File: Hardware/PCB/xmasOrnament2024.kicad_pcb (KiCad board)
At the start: 2 copper layers, 60 x 66.9 mm, 55 parts, among them IC1 TP4056-42, Q1 AO3401A, Q2 CJ3400, SW1 BZCN_TSA007A1518B03, SW2 BZCN_TSA007A1518B03, U1 STM32C011F6

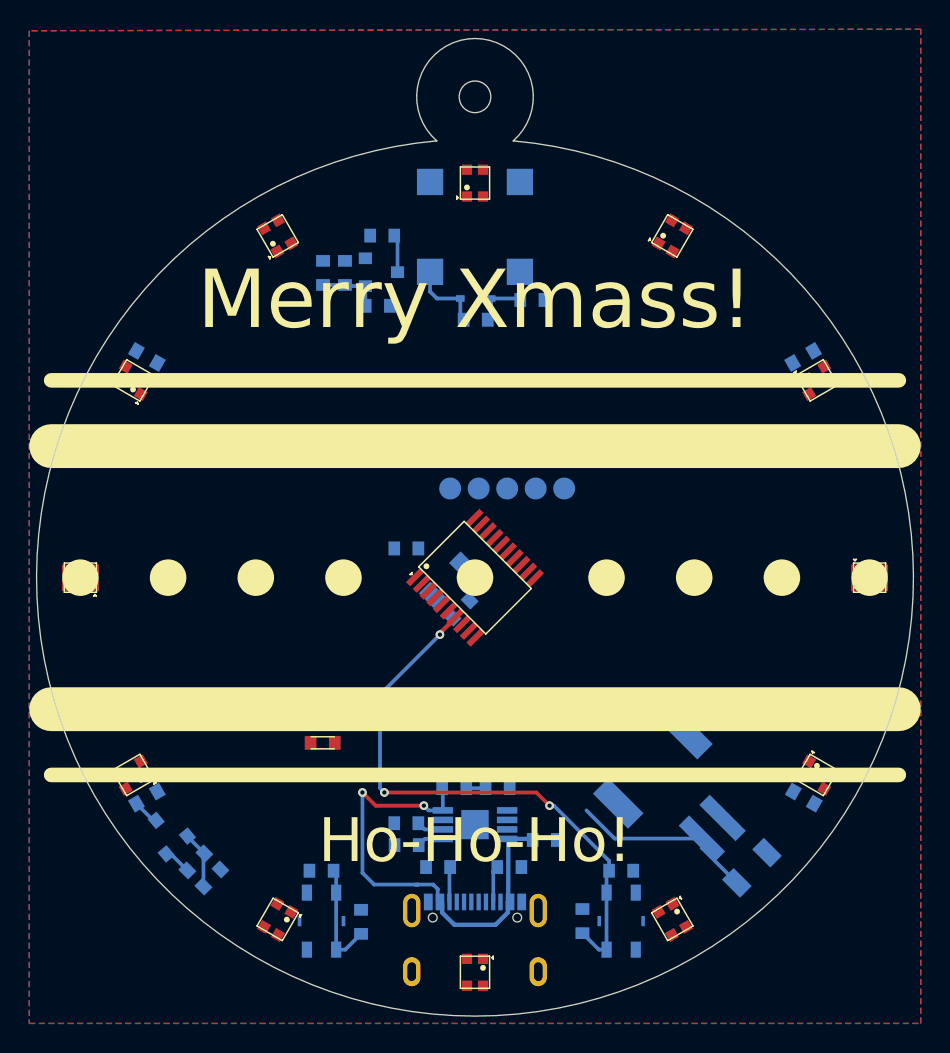
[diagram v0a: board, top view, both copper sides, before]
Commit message: Board finished.
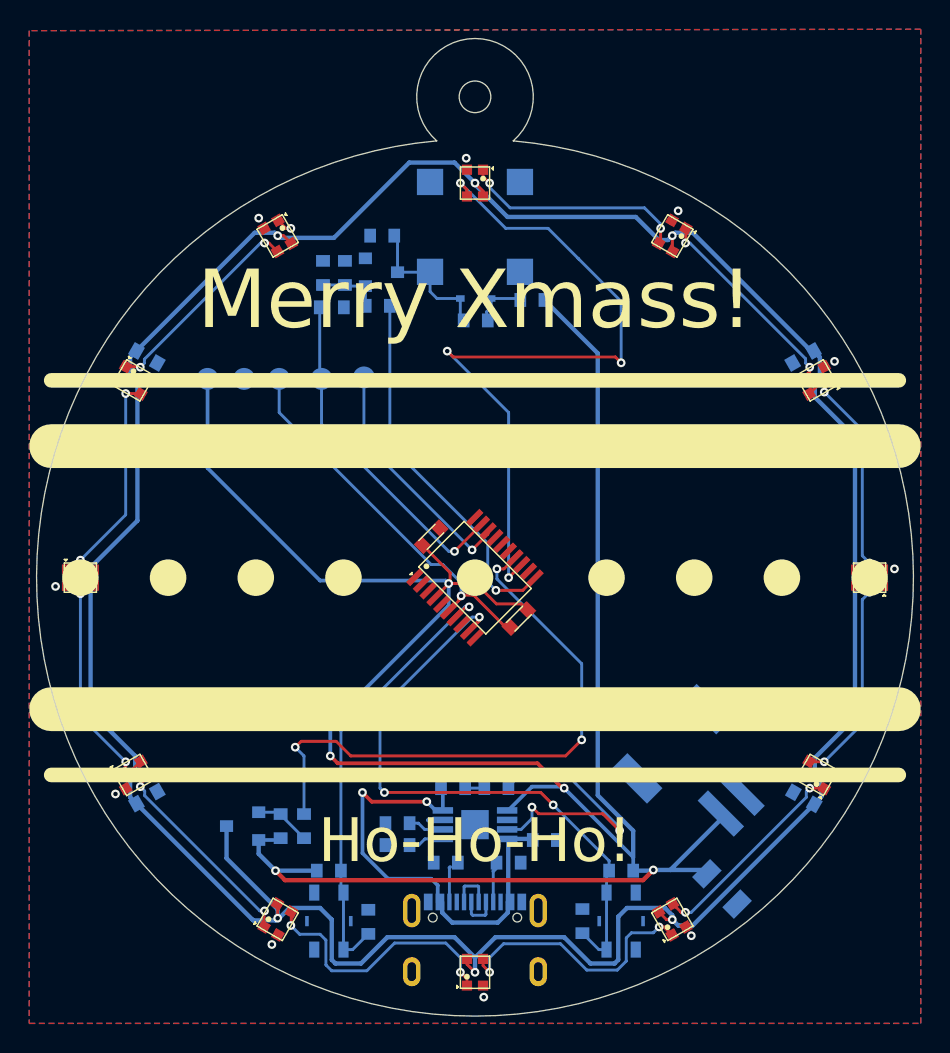
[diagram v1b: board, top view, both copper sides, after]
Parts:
- C4, R13: moved to F.Cu
- R14: moved to B.Cu
- moved R14 29.8 mm to (134.1, 77.2)
- moved TP5 20.9 mm to (130.4, 82.1)
- moved TP2 18.2 mm to (125.5, 82.1)
- moved TP1 17.7 mm to (128.1, 82.1)
- moved TP3 14.7 mm to (133.3, 82.1)
- moved TP4 14.0 mm to (136.2, 82.0)
- moved C3 13.3 mm to (132.3, 105.1), turned to 0 degrees
- moved R7 7.23 mm to (132.2, 112.7), turned to 90 degrees
- moved R6 6.30 mm to (130.6, 112.7), turned to 90 degrees
- moved Q1 5.23 mm to (128.0, 112.7), turned to -90 degrees
- moved R13 4.00 mm to (146.8, 98.5)
- moved C1 2.51 mm to (160.8, 117.0), turned to 135 degrees
- moved CONN1 2.15 mm to (161.4, 111.1)
- moved C4 1.88 mm to (140.8, 92.9), turned to -135 degrees
- moved R2 0.62 mm to (138.6, 114.0)
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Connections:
- C1 pad 2: Net-(IC1-BAT) -> VDD
- CONN1 pad +: Net-(IC1-BAT) -> VDD
- IC1 pad 5: Net-(IC1-BAT) -> VDD
- U1 pad 7: /BTN1 -> /BTN2
- U1 pad 9: /BTN2 -> /BTN1
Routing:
- net WS_SUPPLY: track 1.80 -> 215.0 mm, vias 0 -> 12
- net VDD: track 1.77 -> 165.6 mm, vias 0 -> 5
- net /WS_DIN: track 0.00 -> 50.4 mm, vias 0 -> 4
- net /PERIPH_SUPPLY: track 0.00 -> 41.1 mm, vias 0 -> 3
- net /RST: track 0.00 -> 26.3 mm, vias 0 -> 1
- net /BUZZER: track 0.00 -> 25.5 mm, vias 0 -> 1
- net /SW_CLK: track 0.00 -> 23.4 mm, vias 0 -> 1
- net /BTN2: track 7.62 -> 30.7 mm, vias 0 -> 1
- net Net-(IC1-CHRG): track 0.00 -> 18.9 mm, vias 0 -> 2
- net Net-(LED8-DO): track 0.00 -> 18.1 mm, vias 0 -> 2
- net Net-(LED7-DO): track 0.00 -> 18.1 mm, vias 0 -> 2
- net /SW_DIO: track 0.00 -> 16.6 mm, vias 0 -> 1
- net Net-(LED2-DO): track 0.00 -> 15.5 mm, vias 0 -> 2
- net Net-(LED4-DO): track 0.00 -> 15.1 mm, vias 0 -> 2
- net Net-(LED10-DO): track 0.00 -> 15.0 mm, vias 0 -> 2
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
